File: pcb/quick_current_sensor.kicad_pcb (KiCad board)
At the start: 2 copper layers, 66.2 x 51.8 mm, 25 parts, among them J1 +Vcc, J2 GND, J3 +LOAD, J4 -LOAD, J5 Vout, J6 GND, Q1 MTP2P50E, U1 LM358N, U2 TL431LP

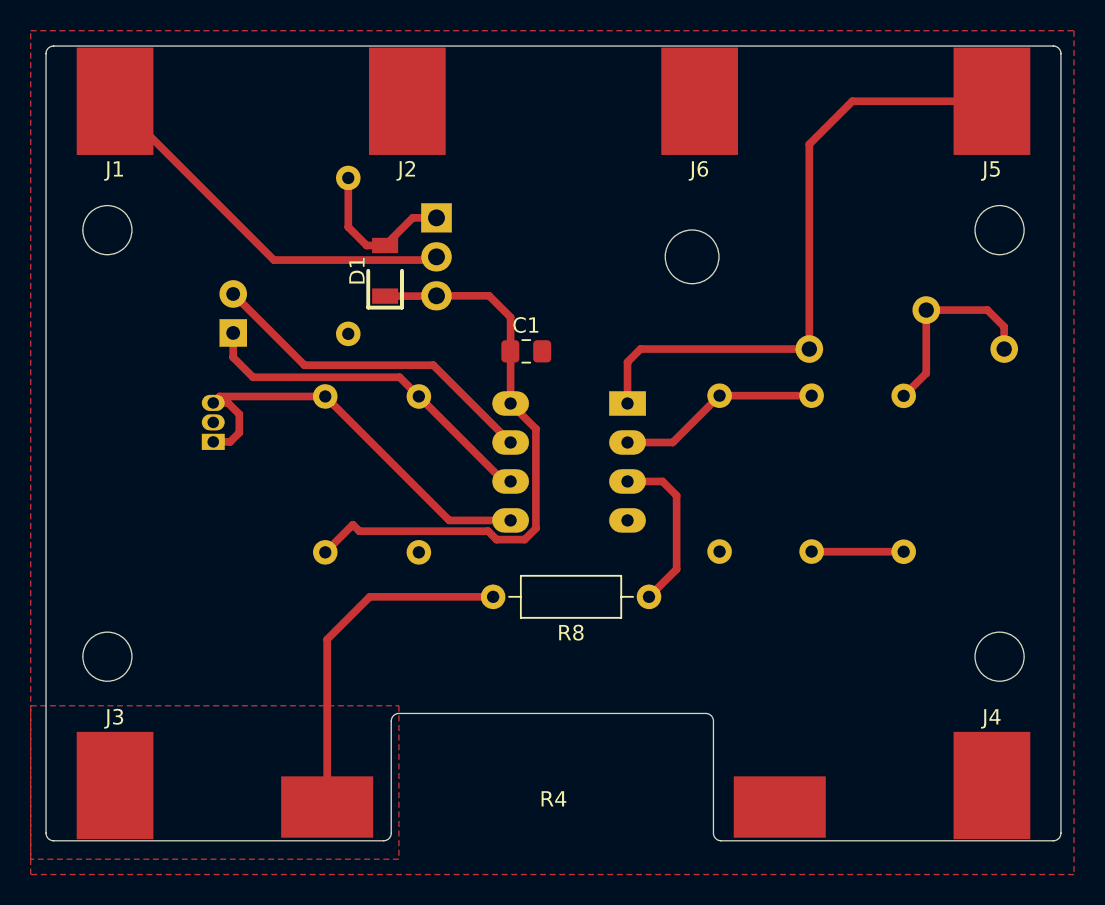
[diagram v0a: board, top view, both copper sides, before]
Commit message: cleanup and add logo
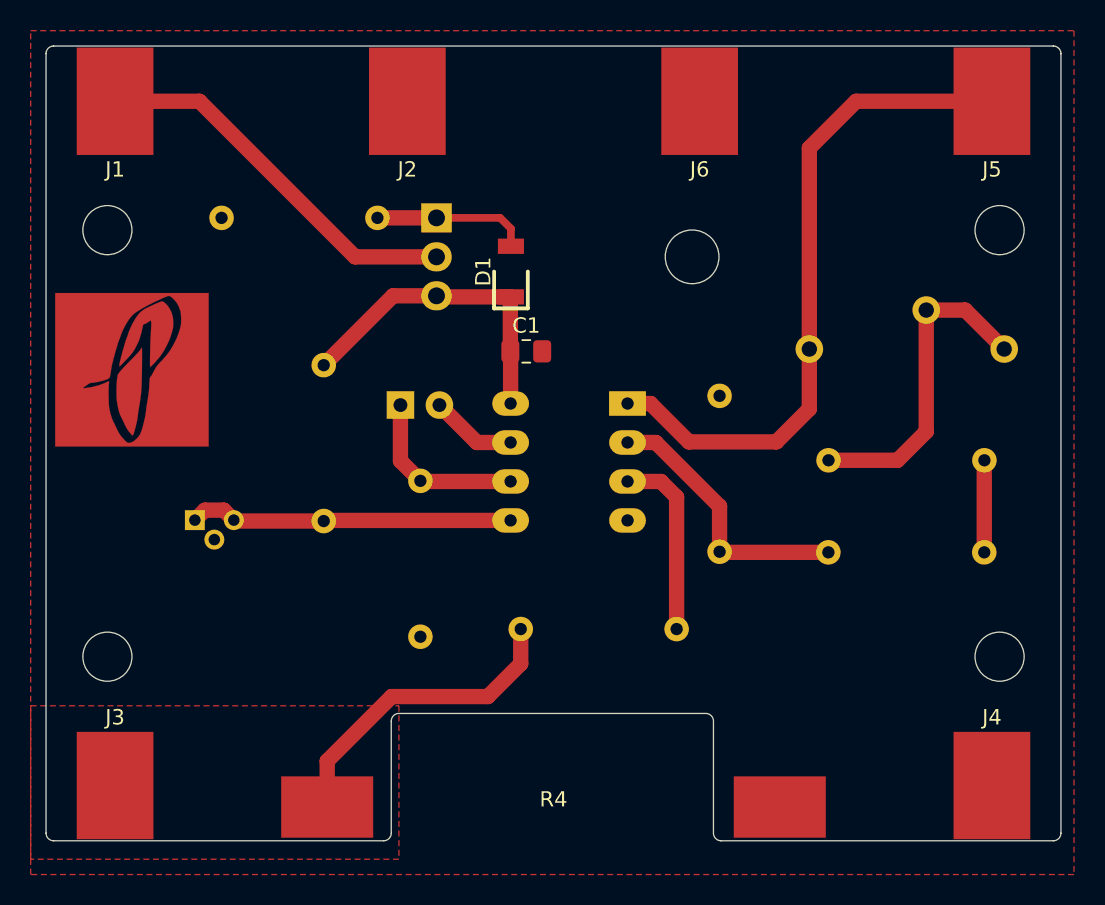
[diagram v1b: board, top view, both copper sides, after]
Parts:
- added G***: LOGO, PL_logo:logoInverse_height_10mm, F.Cu at (85.6, 91.1)
- R8: moved to B.Cu
- U2: footprint Package_TO_SOT_THT:TO-92_Inline -> Package_TO_SOT_THT:TO-92_W4.0mm_StaggerEven_Horizontal_FlatSideDown
- moved R6 12.2 mm to (98.1, 90.8), turned to 270 degrees
- moved D2 11.9 mm to (103.1, 93.4), turned to 0 degrees
- moved R2 11.3 mm to (141.2, 103.0), turned to 180 degrees
- moved R1 10.2 mm to (123.9, 92.8), turned to 270 degrees
- moved D1 8.20 mm to (110.3, 84.7)
- moved R3 6.45 mm to (131.0, 97.0), turned to 0 degrees
- moved R7 5.50 mm to (104.4, 108.5)
- moved U2 5.24 mm to (89.7, 100.9), turned to 0 degrees
- moved R5 3.22 mm to (101.6, 81.2), turned to 180 degrees
- moved R8 2.77 mm to (121.1, 108.0)
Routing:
- net VCC: track 38.4 -> 21.1 mm
- net Net-(D2-Pad2): track 22.1 -> 5.65 mm
- net Net-(D2-Pad1): track 23.0 -> 11.4 mm
- net Net-(R3-Pad1): track 13.2 -> 21.2 mm
- net Net-(R6-Pad2): track 28.1 -> 21.2 mm
- net Net-(R1-Pad2): track 13.3 -> 17.8 mm
- net Net-(J5-Pad1): track 41.3 -> 43.9 mm
- net Net-(J3-Pad1): track 22.9 -> 20.5 mm
- net Net-(R8-Pad1): track 10.9 -> 12.2 mm
